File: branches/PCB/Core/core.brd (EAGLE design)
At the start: 65.7 x 58.4 mm, 20 parts, among them U1 PIC32MX230F064B-

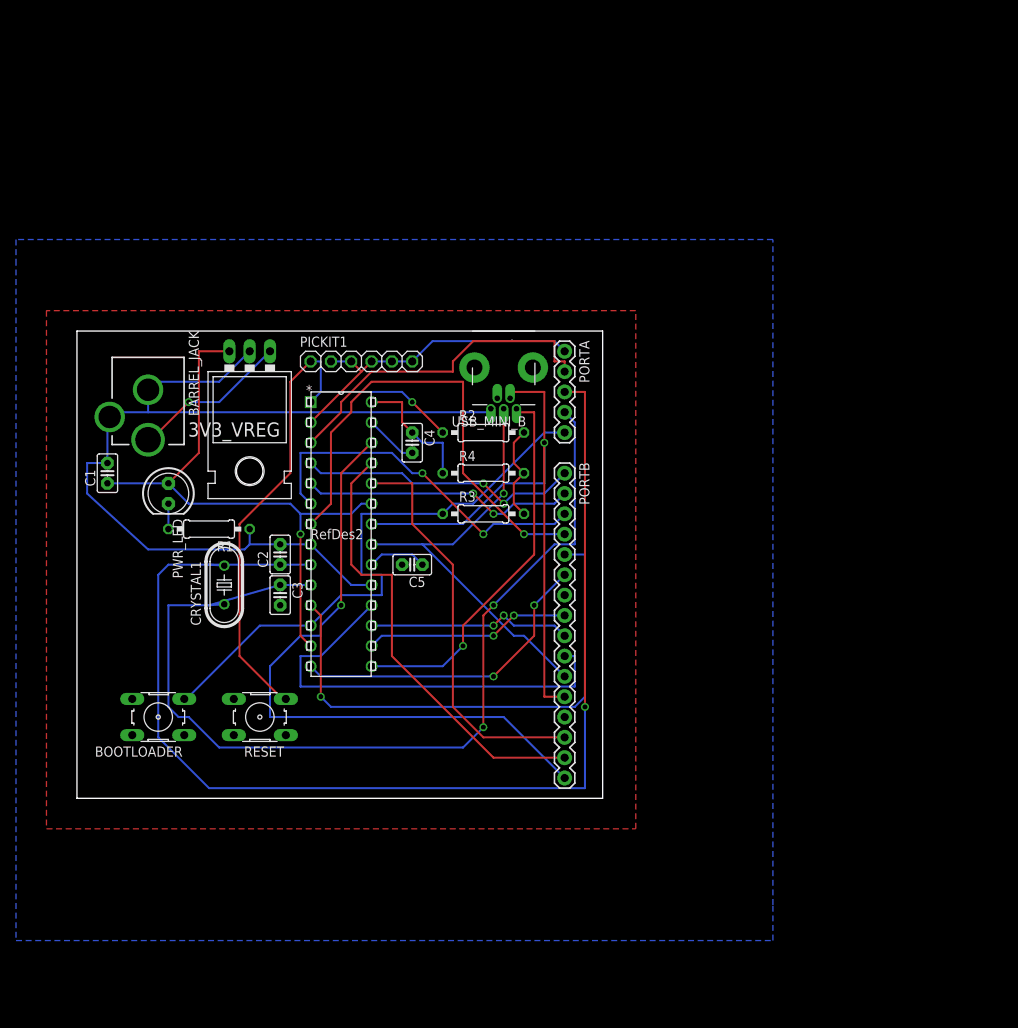
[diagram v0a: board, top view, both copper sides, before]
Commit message: Pre Gerber for Rev 1.00
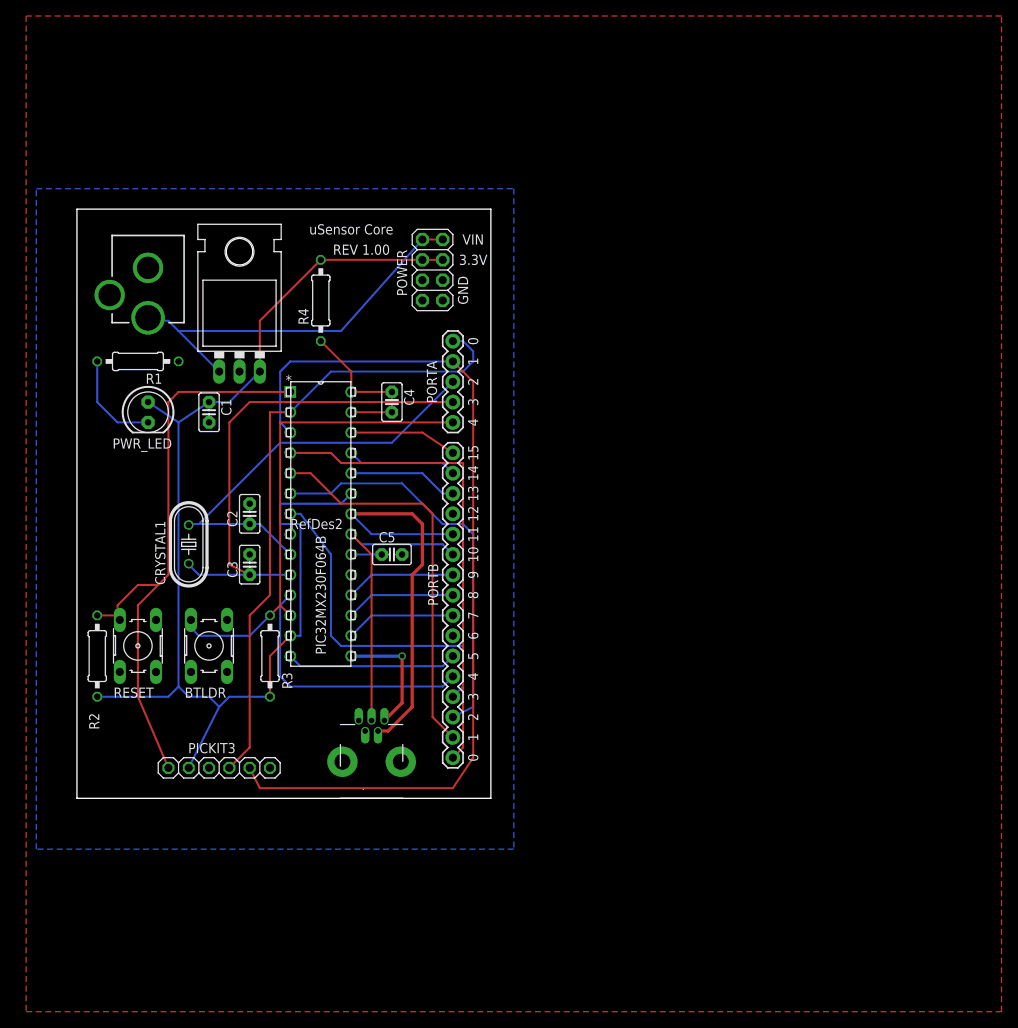
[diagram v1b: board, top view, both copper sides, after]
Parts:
- removed BOOTLOADER: (no value), switch-omron:B3F-10XX
- removed PICKIT1: (no value), adafruit:1X06
- added BTLDR: (no value), switch-omron:B3F-10XX
- added PICKIT3: (no value), adafruit:1X06
- added POWER: (no value), adafruit:2X04
- moved USB_MINI_B 60.7 mm to (36.8, 0.00), turned to 0 degrees
- moved R2 55.8 mm to (2.54, 17.8), turned to 270 degrees
- moved PORTB 38.2 mm to (47.0, 5.08), turned to 90 degrees
- moved R3 32.1 mm to (24.1, 17.8), turned to 270 degrees
- moved R4 29.6 mm to (30.5, 62.2), turned to 90 degrees
- moved R1 22.8 mm to (7.62, 54.6)
- moved RESET 17.6 mm to (7.62, 19.1), turned to 270 degrees
- moved BARREL_JACK 15.2 mm to (8.89, 73.7)
- moved C1 14.8 mm to (16.5, 48.3), turned to 270 degrees
- moved PORTA 14.0 mm to (47.0, 57.1)
- moved PWR_LED 10.5 mm to (8.89, 48.3)
- moved CRYSTAL1 6.75 mm to (14.0, 31.8)
- moved C2 6.35 mm to (21.6, 35.6)
- moved C4 5.68 mm to (39.4, 49.5)
- moved C3 5.39 mm to (21.6, 29.2), turned to 90 degrees
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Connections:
- removed net VDD: 3V3_VREG.OUT, C1.1, PWR_LED.A, U1.13, U1.23
- removed net VSS: 3V3_VREG.GND, BARREL_JACK.GND, BARREL_JACK.GNDBREAK, C1.2, R1.1, U1.19, U1.8, USB_MINI_B.GND
- net +3V3: now also 3V3_VREG.OUT, C1.1, PICKIT3.2, POWER.3, POWER.4, PWR_LED.A, U1.13, U1.23
- net +5V: now also POWER.1, POWER.2
- net D-: now also USB_MINI_B.ID; no longer USB_MINI_B.D-
- net GND: now also 3V3_VREG.GND, BARREL_JACK.GND, BARREL_JACK.GNDBREAK, BTLDR.1, C1.2, PICKIT3.3, POWER.5, POWER.6, POWER.7, POWER.8, R1.1, U1.19, U1.8, USB_MINI_B.VBUS; no longer BOOTLOADER.1
- net MCLR: now also PICKIT3.1; no longer PICKIT1.1
- net RA0: now also PICKIT3.4; no longer PICKIT1.2, PICKIT1.3, PICKIT1.4, PICKIT1.5, PICKIT1.6
- net RA1: now also PICKIT3.5
- net RA4: now also BTLDR.3; no longer BOOTLOADER.3
- net VBUS: now also USB_MINI_B.GND; no longer USB_MINI_B.VBUS
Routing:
- net +3V3: track 12.3 -> 153.1 mm
- net VSS: track 121.5 -> 0.00 mm
- net OSC1: track 149.8 -> 53.5 mm, vias 1 -> 0
- net VDD: track 74.1 -> 0.00 mm, vias 1 -> 0
- net RA1: track 42.3 -> 112.4 mm
- net RB15: track 81.0 -> 13.5 mm, vias 1 -> 0
- net OSC2: track 121.4 -> 63.0 mm, vias 2 -> 0
- net RB14: track 56.4 -> 13.8 mm
- net RB9: track 54.7 -> 13.8 mm
- net RA0: track 40.8 -> 78.9 mm
- net RB13: track 50.7 -> 13.8 mm
- net VBUS: track 48.5 -> 15.3 mm
- net RB4: track 66.3 -> 33.3 mm, vias 1 -> 0
- net +5V: track 20.3 -> 52.3 mm, vias 1 -> 0
- net RB0: track 35.4 -> 59.5 mm, vias 2 -> 0
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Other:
- board size 65.7 x 58.4 mm -> 51.7 x 73.7 mm
- board text added: "0"
- board text added: "1"
- board text added: "10"
- board text added: "11"
- board text added: "12"
- board text added: "13"
- board text added: "14"
- board text added: "15"
- board text added: "2"
- board text added: "3"
- board text added: "3.3V"
- board text added: "4"
- board text added: "5"
- board text added: "6"
- board text added: "7"
- board text added: "8"
- board text added: "9"
- board text added: "GND"
- board text added: "PIC32MX230F064B"
- board text added: "REV 1.00"
- board text added: "VIN"
- board text added: "uSensor Core"
